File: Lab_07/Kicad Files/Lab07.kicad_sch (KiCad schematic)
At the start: 36 parts, among them J101 Conn_01x01_Socket, J102 Conn_01x01_Socket, J103 0, J104 Output_Terminal, J301 Conn_01x01_Socket, J302 Conn_01x01_Socket, J303 Output_Terminal, J304 0, Q101 NPN, Q102 TIP120, Q301 NPN, Q302 PMOS, Q303 NPN

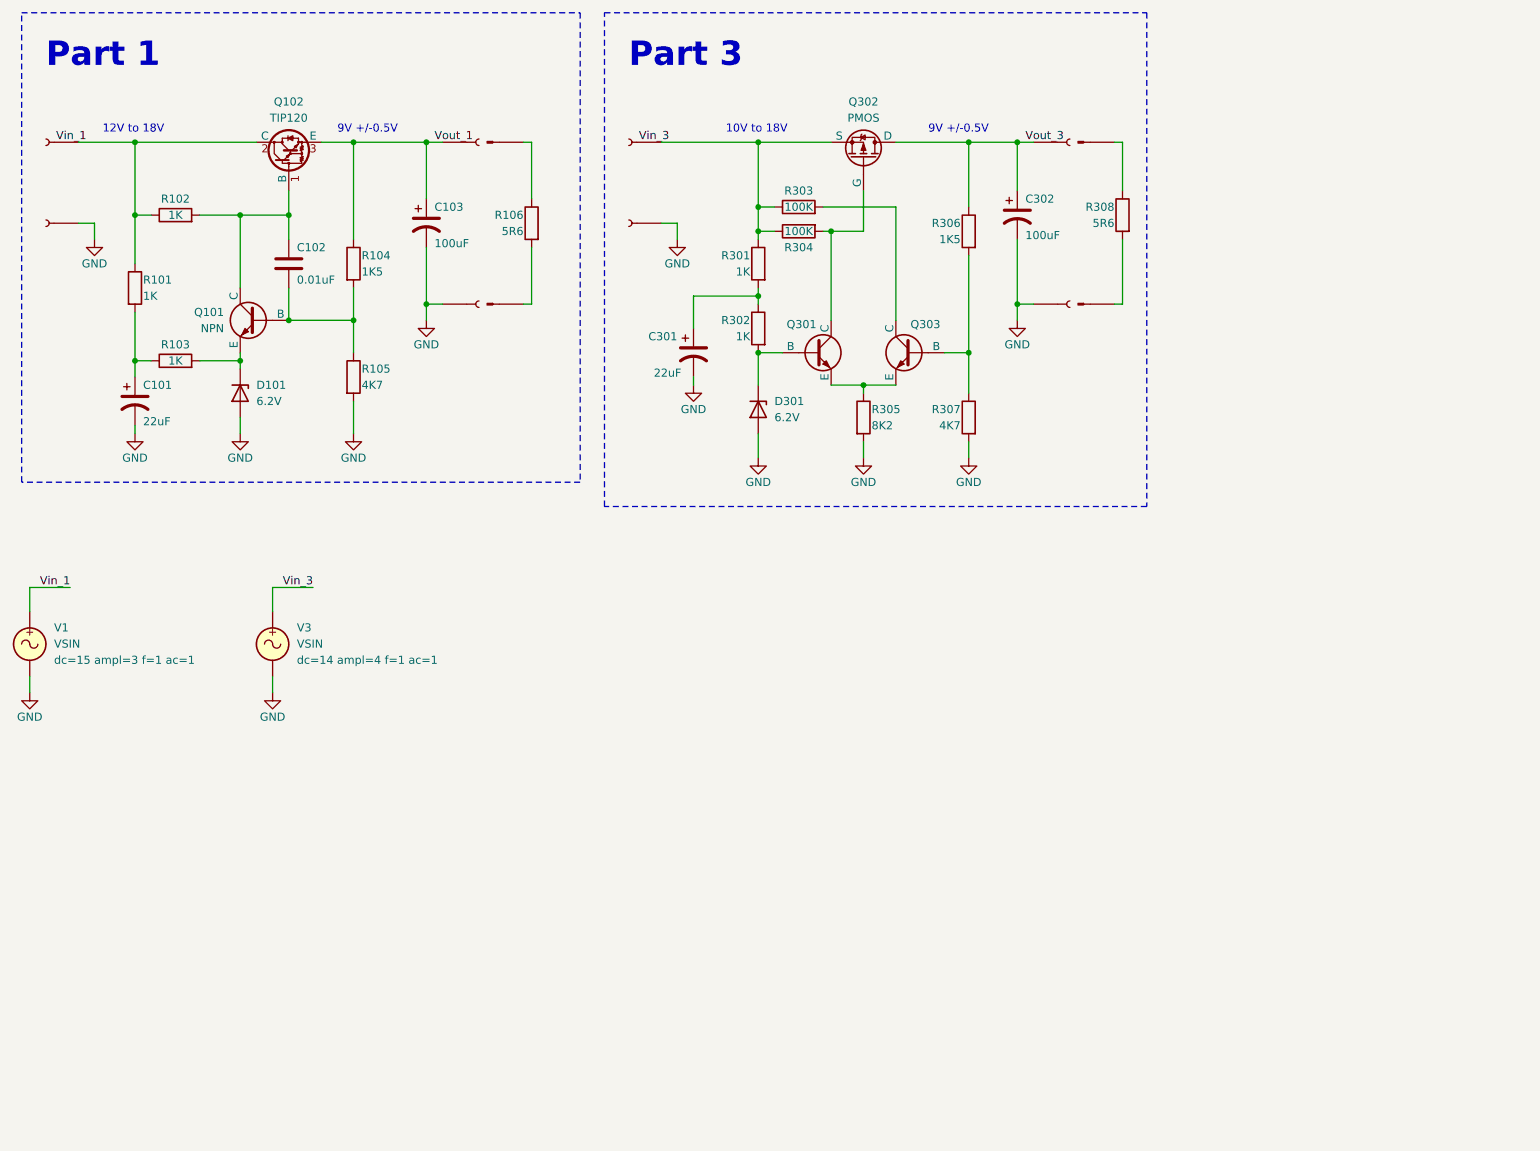
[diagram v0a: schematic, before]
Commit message: Finish Lab 7
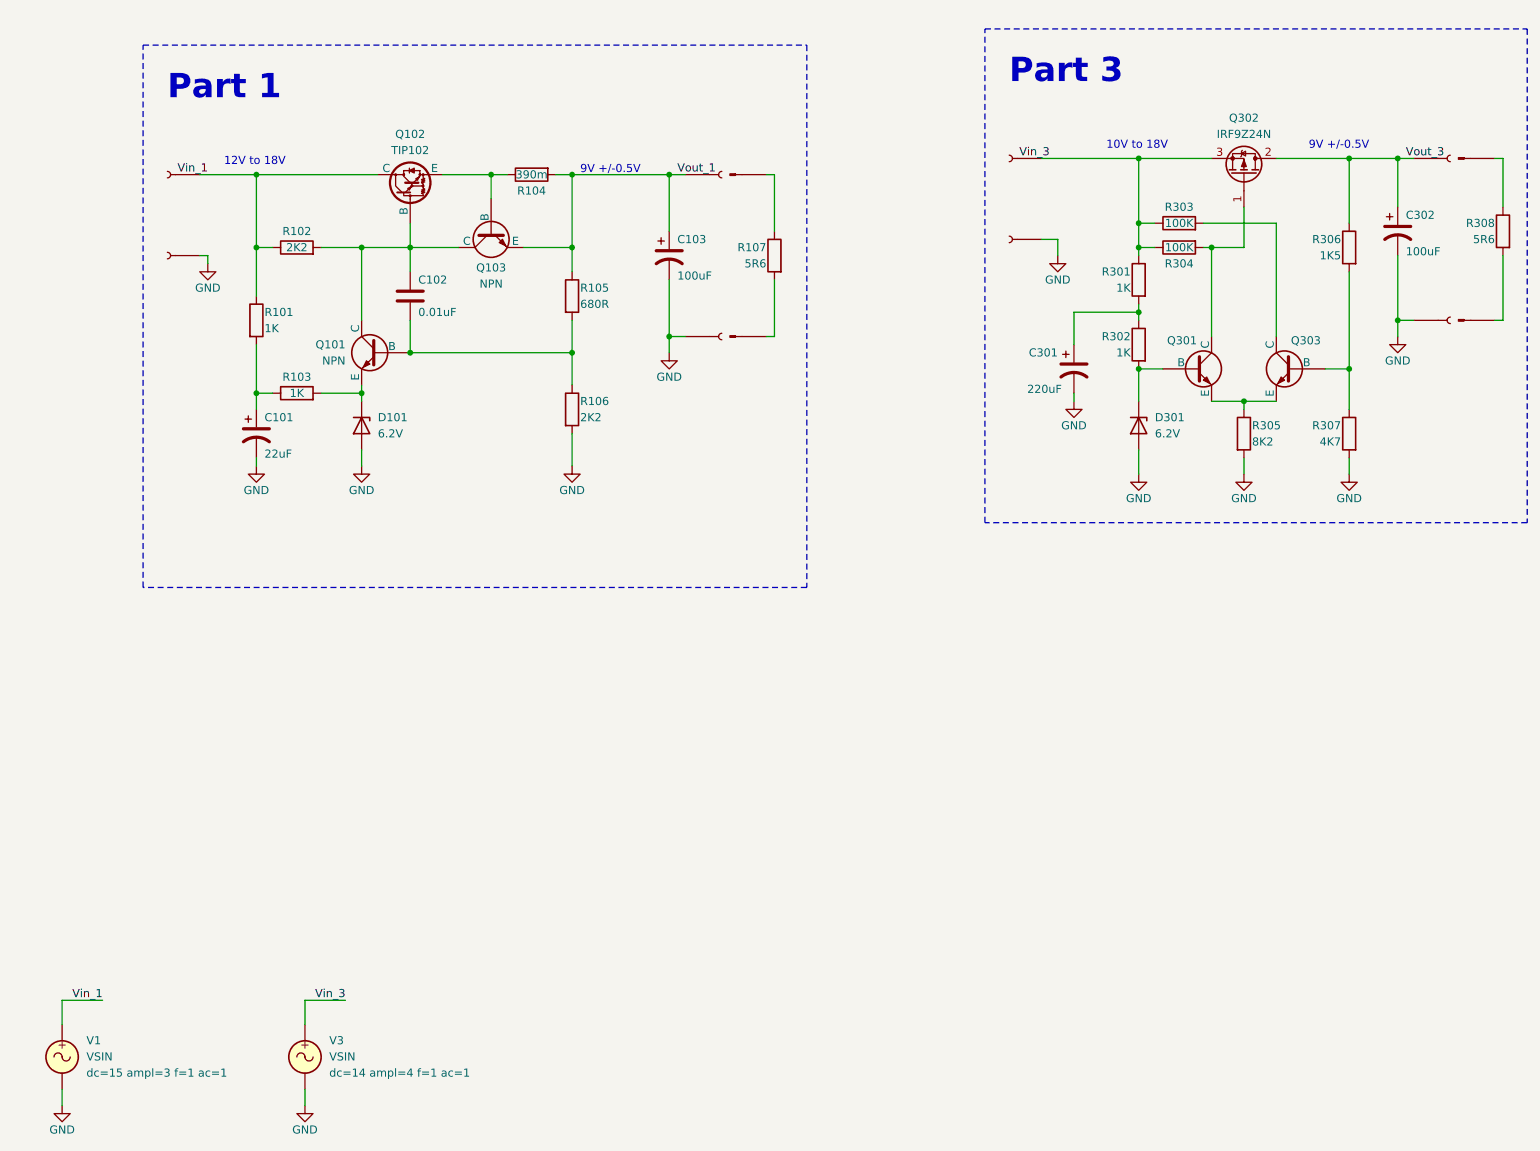
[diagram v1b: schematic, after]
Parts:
- added Q103: NPN, Package_TO_SOT_THT:TO-92L_Inline_Wide, symbol Transistor_BJT:2N3904
- added R104: 390m, Resistor_THT:R_Axial_DIN0207_L6.3mm_D2.5mm_P2.54mm_Vertical, symbol Device:R
- C101, C103, C302: footprint (none) -> Capacitor_THT:CP_Radial_D10.0mm_P5.00mm
- C102: footprint (none) -> Capacitor_THT:C_Disc_D10.0mm_W2.5mm_P5.00mm
- C301: value 22uF -> 220uF; footprint (none) -> Capacitor_THT:CP_Radial_D10.0mm_P5.00mm
- D101, D301: footprint (none) -> Diode_THT:D_DO-41_SOD81_P7.62mm_Horizontal
- J101, J102, J103, J104, J301, J302, J303, J304: footprint (none) -> TestPoint:TestPoint_Loop_D2.54mm_Drill1.5mm_Beaded
- Q101, Q301, Q303: footprint (none) -> Package_TO_SOT_THT:TO-92L_Inline_Wide; symbol Simulation_SPICE:NPN -> Transistor_BJT:2N3904
- Q102: value TIP120 -> TIP102
- Q302: value PMOS -> IRF9Z24N; footprint (none) -> Package_TO_SOT_THT:TO-220-3_Vertical; symbol Device:Q_PMOS_DGS -> Device:Q_PMOS_GDS
- R101, R103, R301, R302, R303, R304, R305, R306, R307: footprint (none) -> Resistor_THT:R_Axial_DIN0207_L6.3mm_D2.5mm_P7.62mm_Horizontal
- R102: value 1K -> 2K2; footprint (none) -> Resistor_THT:R_Axial_DIN0207_L6.3mm_D2.5mm_P7.62mm_Horizontal
- R105: renamed from R104; value 1K5 -> 680R; footprint (none) -> Resistor_THT:R_Axial_DIN0207_L6.3mm_D2.5mm_P7.62mm_Horizontal
- R106: renamed from R105; value 4K7 -> 2K2; footprint (none) -> Resistor_THT:R_Axial_DIN0207_L6.3mm_D2.5mm_P7.62mm_Horizontal
- V1, V3: now left out of the parts list
- renumbered R106 to R107
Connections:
- net Vout_1: now also Q103.1 (E), R104.2; no longer Q102.3 (E)
- net Vout_3: now also Q302.2 (D); no longer Q302.1 (D)
- net at C102.1, Q102.1 (B), R102.2: now also Q101.3 (C), Q103.3 (C); no longer Q101.1 (C)
- net at D101.1 (K), R103.2: now also Q101.1 (E); no longer Q101.3 (E)
- net at R303.2: now also Q303.3 (C); no longer Q303.1 (C)
- new net: Q301.3 (C), Q302.1 (G), R304.2
- new net: Q102.3 (E), Q103.2 (B), R104.1
- new net: Q301.1 (E), Q303.1 (E), R305.1
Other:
- moved on the sheet: C101, C102, C103, C301, C302, D101, D301, Q302, R101, R102, R103, R105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
